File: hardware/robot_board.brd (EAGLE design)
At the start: 95.2 x 76.1 mm, 147 parts, among them J1 POWER_JACKPTH, Q1 DMP2035U, Q2 DMP2035U, Q3 DMP2035U-7, Q4 DMP2035U-7, U1 FT232RL-BASICSSOP, U11 LM393, U12 LM393, U16 LM393, U17 ATMEGA325PA, U2 SIA907EDJT, U3 MIC5219, U4 HC_05, U5 SIA907EDJT, U6 SIA907EDJT, U7 TLV70233, Y1 16MHz

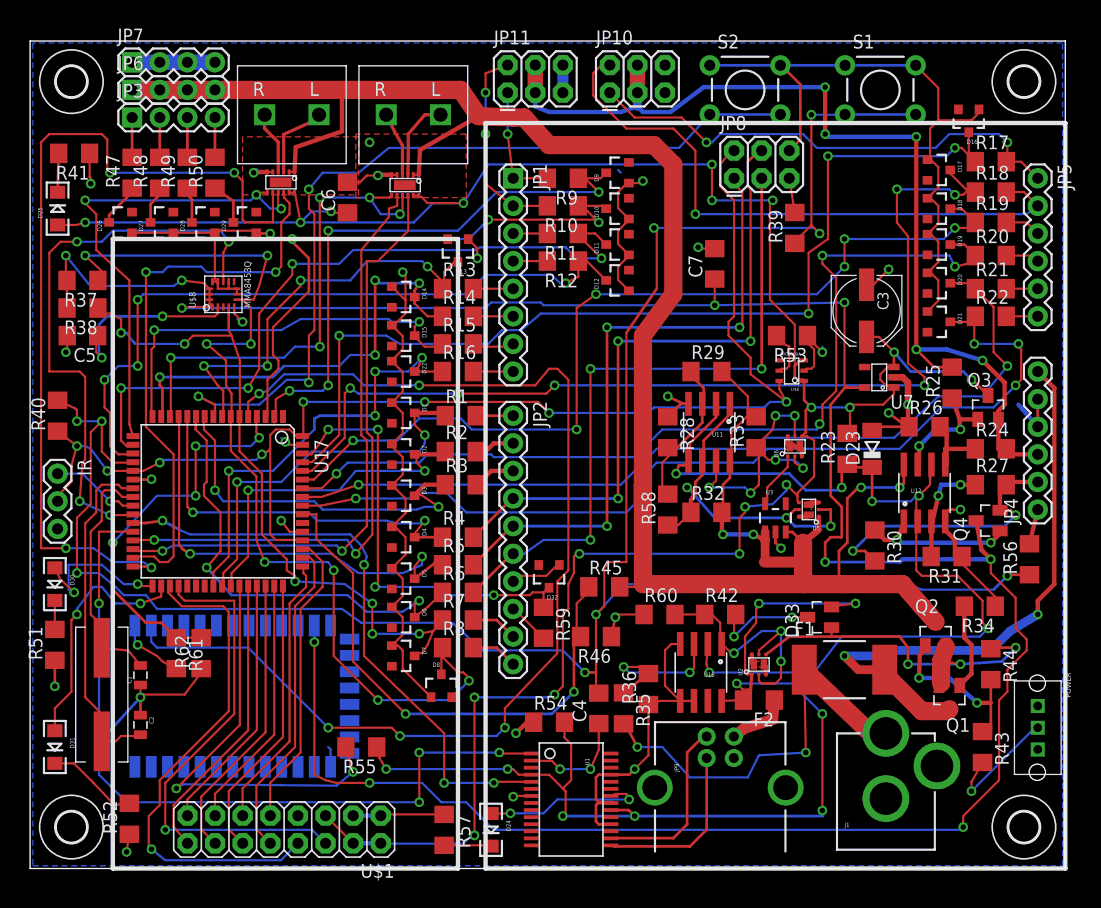
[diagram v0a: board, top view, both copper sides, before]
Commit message: updated routing
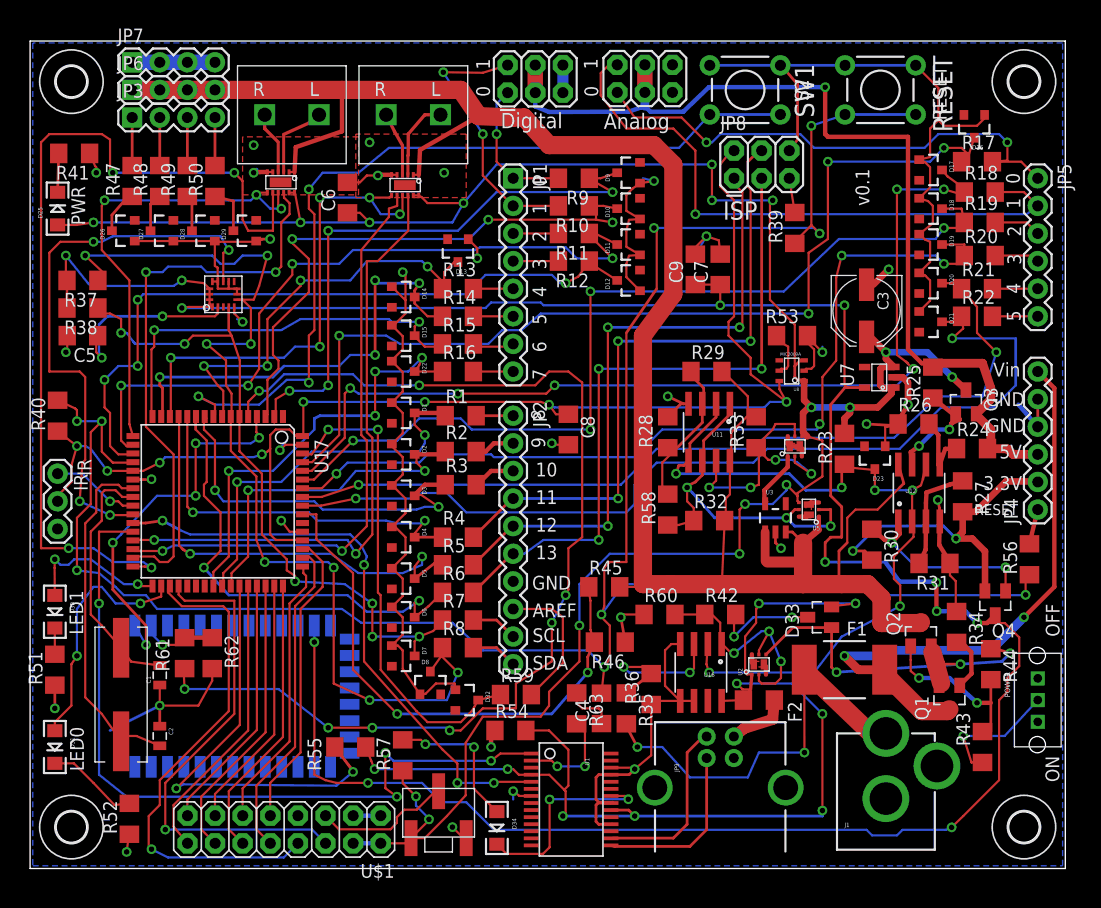
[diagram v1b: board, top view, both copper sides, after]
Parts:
- removed D24: POWER, SparkFun-LED:LED-1206
- added C8: .1uF, resistor:C1206
- added C9: 1uF, resistor:C1206
- added D34: POWER, SparkFun-LED:LED-1206
- added R63: 1K, resistor:R1206
- added U$2: POT, r_cubed:POT
- D23: value 2.1V -> 2.4V; device diode:SOD80C -> SparkFun-DiscreteSemi:SOT23-3
- R24: value 12K -> 12K 1%
- R26: value 7.68K -> 7.68K 1%
- R27, R28, R45, R46: value 10K -> 10K 1%
- R29, R31: value 15K -> 15K 1%
- R58: value 300K -> 300K 1%
- moved D32 13.7 mm to (40.1, 15.5), turned to 270 degrees
- moved R57 7.85 mm to (34.3, 10.4), turned to 90 degrees
- moved Q4 7.60 mm to (88.8, 24.4), turned to 180 degrees
- moved R59 7.08 mm to (44.7, 16.0), turned to 0 degrees
- moved R54 3.64 mm to (44.2, 12.7)
- moved R34 2.86 mm to (85.2, 22.2), turned to 270 degrees
- moved R27 2.80 mm to (85.8, 34.2), turned to 270 degrees
- moved D30 2.54 mm to (2.29, 23.6)
- moved POWER 2.54 mm to (92.7, 15.5)
- moved R51 2.29 mm to (2.29, 18.3)
- moved Q3 2.09 mm to (86.1, 42.9)
- moved C2 2.05 mm to (11.9, 12.2)
- moved C1 1.78 mm to (11.9, 17.8)
- moved Y1 1.78 mm to (8.38, 16.0)
- moved R25 1.78 mm to (83.1, 44.7)
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- renumbered S1 to RESET, U$4 to U9, U$5 to U10, U$6 to U8
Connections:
- new net N$13: R61.1, R62.2, U4.2
- new net N$15: U$1.5, U$2.2
- net 2.1V: now also D23.3; no longer D23.C
- net 3V3: now also C9.1
- net 5V: now also R57.1, U$2.1; no longer U$1.5
- net 5V_UC: now also C8.1
- net BT_RX: now also R61.2; no longer U4.2
- net BT_TX: now also U4.1; no longer R61.1, R62.2
- net DTR: now also R63.1; no longer U1.2
- net GND: now also C8.2, C9.2, D23.1, U$2.3, U1.26; no longer D23.A, R57.1
- net N$10: now also D34.C; no longer D24.A
- net N$11: now also D34.A; no longer D24.C
- net N$14: now also R63.2, U1.2; no longer R61.2, U4.1
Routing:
- net 2.1V: track 87.3 -> 71.8 mm
- net N$15: track 0.00 -> 12.7 mm
- net N$11: track 4.35 -> 13.6 mm, vias 0 -> 2
- net AREF: track 3.91 -> 13.1 mm
- net N$13: track 0.00 -> 7.05 mm, vias 0 -> 1
- net GND: track 301.4 -> 308.4 mm, vias 28 -> 32
- net D1: track 18.7 -> 24.7 mm
- net DTR: track 10.1 -> 4.66 mm, vias 2 -> 0
- net 3V3_OUT: track 26.5 -> 30.8 mm
- net AREF_IN: track 40.7 -> 44.6 mm, vias 4 -> 2
- net BT_RX: track 105.6 -> 101.8 mm, vias 5 -> 8
- net N$10: track 15.3 -> 18.8 mm
- net N$45: track 14.9 -> 18.3 mm
- net 3V3: track 241.7 -> 238.4 mm, vias 10 -> 12
- net N$14: track 6.09 -> 9.37 mm, vias 1 -> 2
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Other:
- board text added: "0"
- board text added: "1"
- board text added: "10"
- board text added: "11"
- board text added: "12"
- board text added: "13"
- board text added: "2"
- board text added: "3"
- board text added: "3.3V"
- board text added: "4"
- board text added: "5"
- board text added: "5V"
- board text added: "6"
- board text added: "7"
- board text added: "8"
- board text added: "9"
- board text added: "AREF"
- board text added: "Analog"
- board text added: "Digital"
- board text added: "GND"
- board text added: "IR"
- board text added: "ISP"
- board text added: "LED0"
- board text added: "LED1"
- board text added: "OFF"
- board text added: "ON"
- board text added: "PWR"
- board text added: "RESET"
- board text added: "SCL"
- board text added: "SDA"
- board text added: "SW1"
- board text added: "Vin"
- board text added: "v0.1"
